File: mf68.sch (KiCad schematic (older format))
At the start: 1 part, among them U1 nice_nano

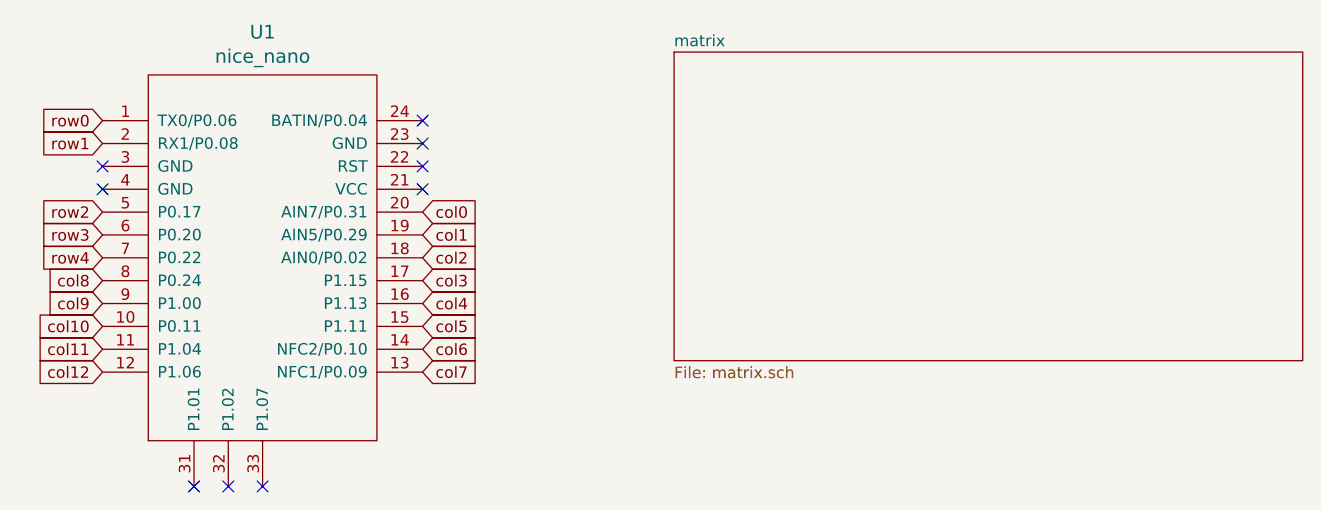
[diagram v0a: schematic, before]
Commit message: Wip: row stagger is wrong!
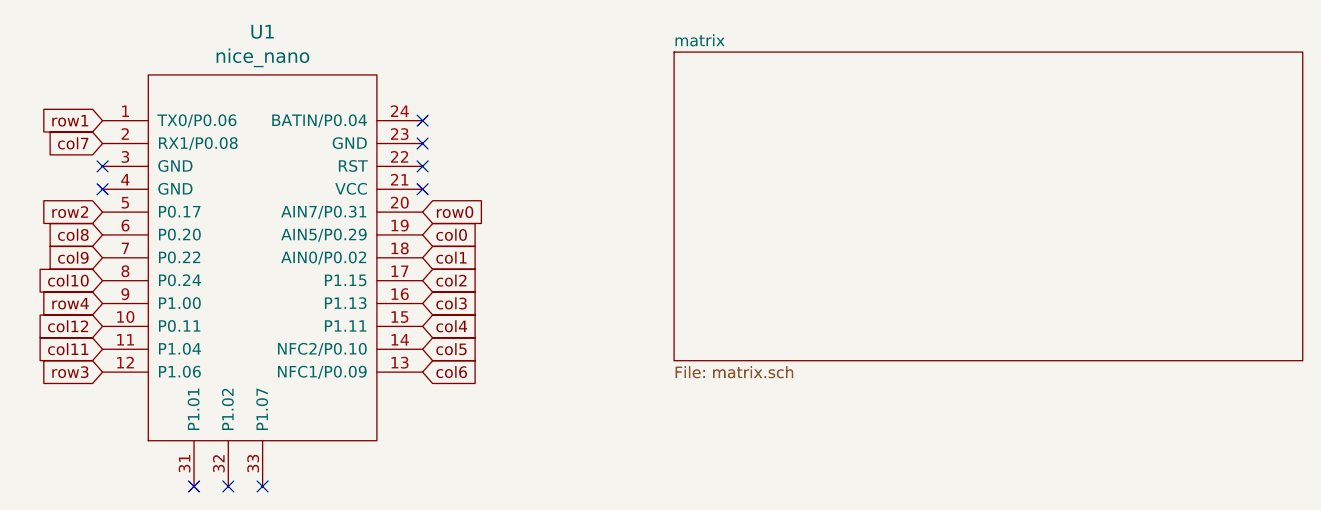
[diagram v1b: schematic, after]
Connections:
- net col0: now also U1.19 (AIN5/P0.29); no longer U1.20 (AIN7/P0.31)
- net col1: now also U1.18 (AIN0/P0.02); no longer U1.19 (AIN5/P0.29)
- net col10: now also U1.8 (P0.24); no longer U1.10 (P0.11)
- net col12: now also U1.10 (P0.11); no longer U1.12 (P1.06)
- net col2: now also U1.17 (P1.15); no longer U1.18 (AIN0/P0.02)
- net col3: now also U1.16 (P1.13); no longer U1.17 (P1.15)
- net col4: now also U1.15 (P1.11); no longer U1.16 (P1.13)
- net col5: now also U1.14 (NFC2/P0.10); no longer U1.15 (P1.11)
- net col6: now also U1.13 (NFC1/P0.09); no longer U1.14 (NFC2/P0.10)
- net col7: now also U1.2 (RX1/P0.08); no longer U1.13 (NFC1/P0.09)
- net col8: now also U1.6 (P0.20); no longer U1.8 (P0.24)
- net col9: now also U1.7 (P0.22); no longer U1.9 (P1.00)
- net row0: now also U1.20 (AIN7/P0.31); no longer U1.1 (TX0/P0.06)
- net row1: now also U1.1 (TX0/P0.06); no longer U1.2 (RX1/P0.08)
- net row3: now also U1.12 (P1.06); no longer U1.6 (P0.20)
- net row4: now also U1.9 (P1.00); no longer U1.7 (P0.22)
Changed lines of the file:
@@
 $EndSheet
 Text GLabel 1450 2350 0    50   Input ~ 0
-row0
-Text GLabel 1450 2450 0    50   Input ~ 0
 row1
 Text GLabel 1450 2750 0    50   Input ~ 0
 row2
-Text GLabel 1450 2850 0    50   Input ~ 0
+Text GLabel 1450 3450 0    50   Input ~ 0
 row3
-Text GLabel 1450 2950 0    50   Input ~ 0
+Text GLabel 1450 3150 0    50   Input ~ 0
 row4
-Text GLabel 2850 2750 2    50   Input ~ 0
+Text GLabel 2850 2850 2    50   Input ~ 0
 col0
-Text GLabel 2850 2850 2    50   Input ~ 0
+Text GLabel 2850 2950 2    50   Input ~ 0
 col1
-Text GLabel 2850 2950 2    50   Input ~ 0
+Text GLabel 2850 3050 2    50   Input ~ 0
 col2
-Text GLabel 2850 3050 2    50   Input ~ 0
+Text GLabel 2850 3150 2    50   Input ~ 0
 col3
-Text GLabel 2850 3150 2    50   Input ~ 0
-col4
-Text GLabel 2850 3250 2    50   Input ~ 0
-col5
-Text GLabel 2850 3350 2    50   Input ~ 0
-col6
-Text GLabel 2850 3450 2    50   Input ~ 0
+Text GLabel 1450 2450 0    50   Input ~ 0
 col7
 NoConn ~ 1450 2550
@@
 NoConn ~ 2000 3950
 NoConn ~ 1850 3950
-Text GLabel 1450 3450 0    50   Input ~ 0
+Text GLabel 1450 3250 0    50   Input ~ 0
 col12
 Text GLabel 1450 3350 0    50   Input ~ 0
 col11
-Text GLabel 1450 3250 0    50   Input ~ 0
+Text GLabel 1450 3050 0    50   Input ~ 0
 col10
-Text GLabel 1450 3150 0    50   Input ~ 0
+Text GLabel 1450 2950 0    50   Input ~ 0
 col9
-Text GLabel 1450 3050 0    50   Input ~ 0
+Text GLabel 1450 2850 0    50   Input ~ 0
 col8
+Text GLabel 2850 2750 2    50   Input ~ 0
+row0
+Text GLabel 2850 3250 2    50   Input ~ 0
+col4
+Text GLabel 2850 3450 2    50   Input ~ 0
+col6
+Text GLabel 2850 3350 2    50   Input ~ 0
+col5
 $EndSCHEMATC
